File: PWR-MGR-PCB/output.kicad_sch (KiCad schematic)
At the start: 7 parts, among them J1 Conn_01x02_Pin, J2 Conn_01x02_Pin, J5 Conn_01x02_Pin

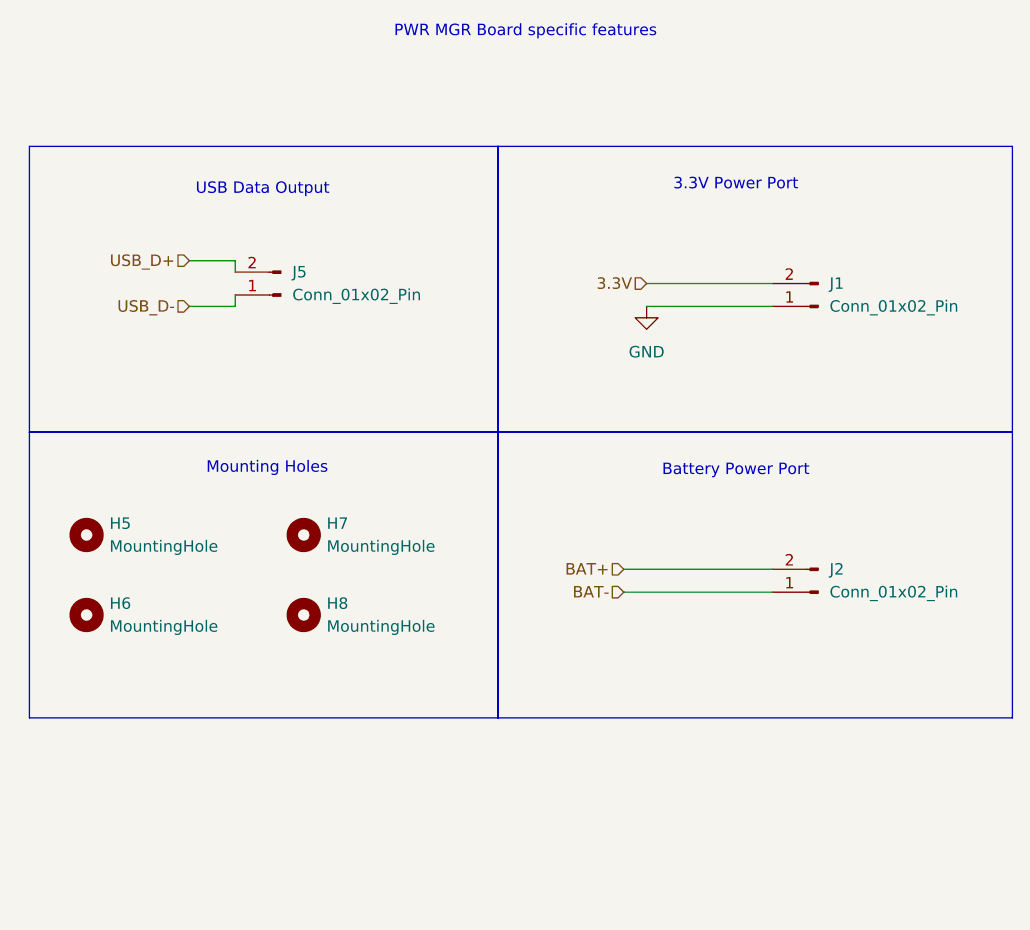
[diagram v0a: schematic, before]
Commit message: begin v2, update schematic
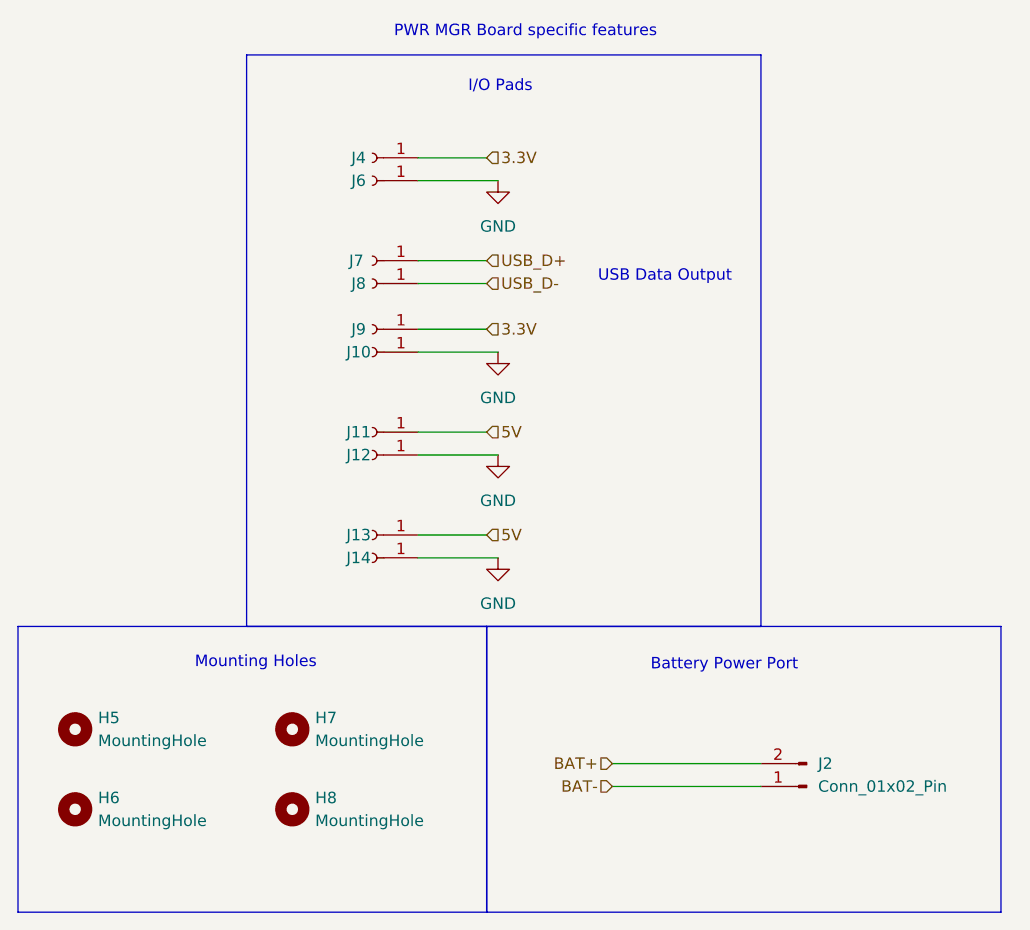
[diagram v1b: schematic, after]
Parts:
- removed J1: Conn_01x02_Pin, Connector_JST:JST_XH_B2B-XH-A_1x02_P2.50mm_Vertical, symbol Connector:Conn_01x02_Pin
- removed J5: Conn_01x02_Pin, Connector_PinHeader_2.00mm:PinHeader_1x02_P2.00mm_Vertical, symbol Connector:Conn_01x02_Pin
- added J10, J11, J12, J13, J14, J4, J6, J7, J8, J9: Conn_01x01_Socket, Custom_Footprints:Drilled_Solder_Pad_0.6mm_3x1mm, symbol Connector:Conn_01x01_Socket
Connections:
- net 3.3V: now also J4.1 (Pin_1), J9.1 (Pin_1)
- net GND: now also J10.1 (Pin_1), J12.1 (Pin_1), J14.1 (Pin_1), J6.1 (Pin_1)
- net USB_D+: now also J7.1 (Pin_1)
- net USB_D-: now also J8.1 (Pin_1)
- new net 5V: J11.1 (Pin_1), J13.1 (Pin_1)
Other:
- note added: "I/O Pads"
- note removed: "3.3V Power Port"
- moved on the sheet: H5, H6, H7, H8, J2
